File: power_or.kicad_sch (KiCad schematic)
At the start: 3 parts, among them Q1 AO3401A

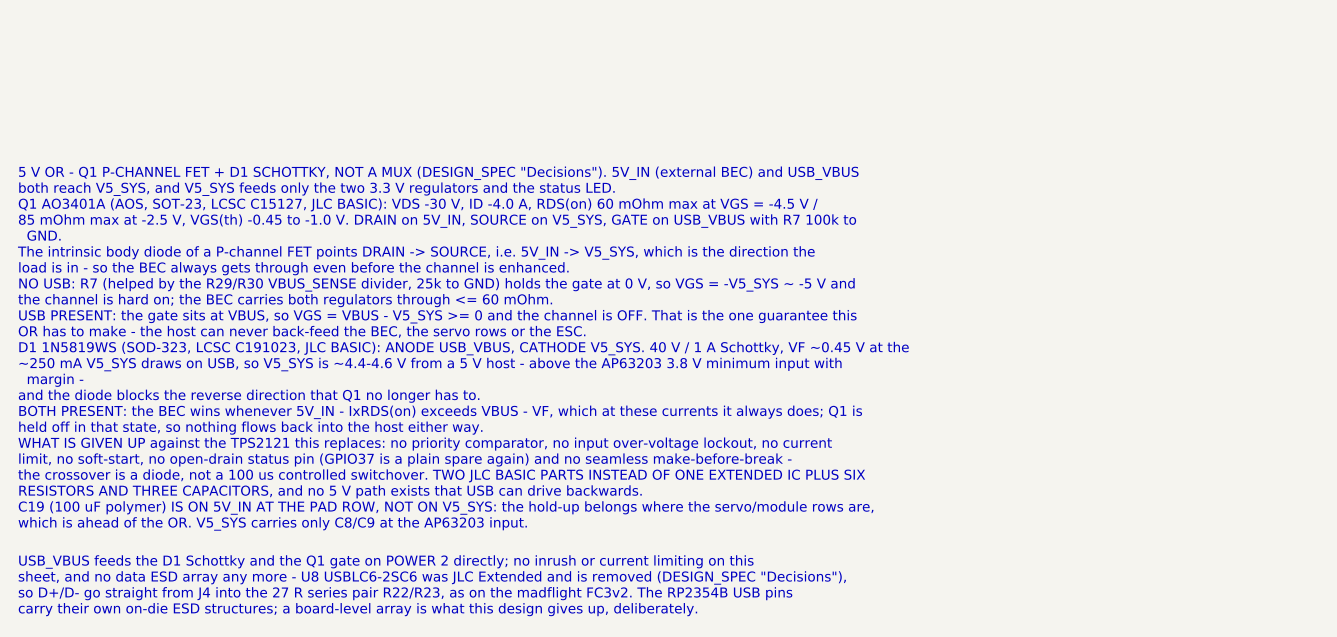
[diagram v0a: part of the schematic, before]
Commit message: updoot
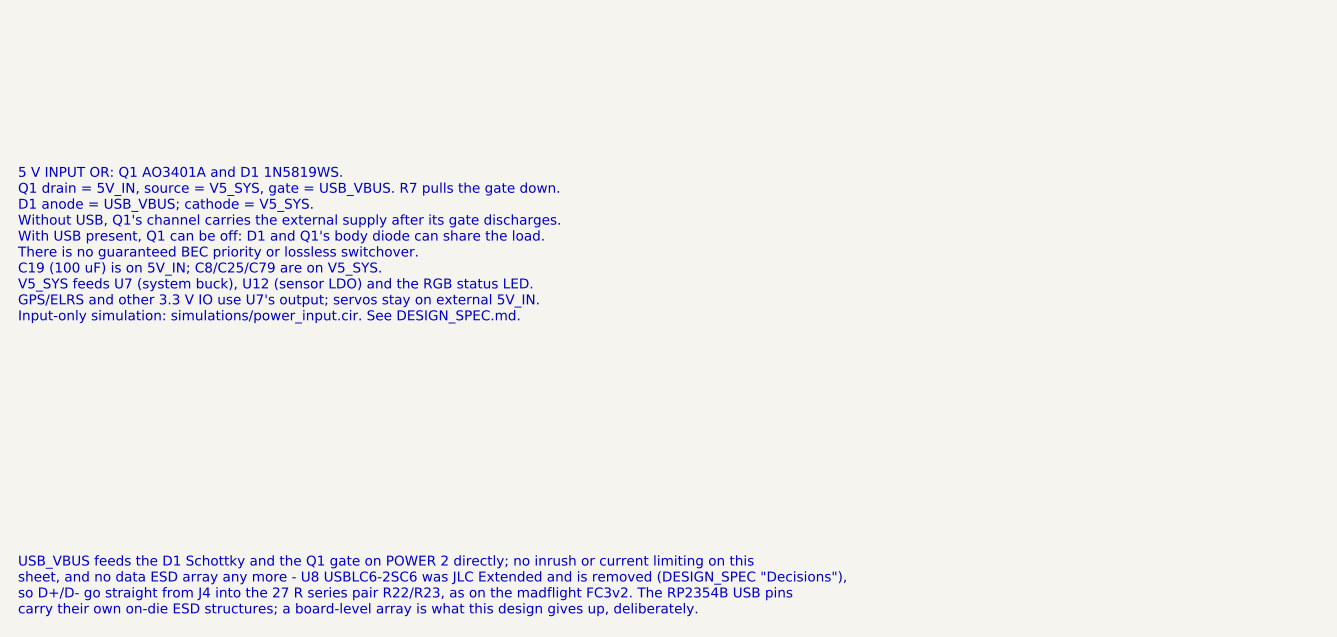
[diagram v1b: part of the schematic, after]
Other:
- note added: "5 V INPUT OR: Q1 AO3401A and D1 1N5819WS. Q1 drain = 5V_IN, source = V5_SYS, gate = USB_VBUS. R7 pulls the gate down. D1 anode = USB_VBUS; cathode = V5_SYS. Without USB, Q1's channel carries the external supply after its gate discharges. With USB present, Q1 can be off: D1 and Q1's body diode can share the load. There is no guaranteed BEC priority or lossless switchover. C19 (100 uF) is on 5V_IN;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"
- note removed: "5 V OR - Q1 P-CHANNEL FET + D1 SCHOTTKY, NOT A MUX (DESIGN_SPEC "Decisions"). 5V_IN (external BEC) and USB_VBUS both reach V5_SYS, and V5_SYS feeds only the two 3.3 V regulators and the status LED. Q1 AO3401A (AOS, SOT-23, LCSC C15127, JLC BASIC): VDS -30 V, ID -4.0 A, RDS(on) 60 mOhm max at VGS = -4.5 V / 85 mOhm max at -2.5 V, VGS(th) -0.45 to -1.0 V. DRAIN on 5V_IN, SOURCE on V5_SYS, GATE on U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"
